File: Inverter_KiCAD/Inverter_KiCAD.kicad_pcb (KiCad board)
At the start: 2 copper layers, 184 x 186 mm, 172 parts, among them J101 Conn_02x19_Odd_Even, J102 Conn_01x03, J103 Conn_02x19_Odd_Even, J104 Conn_01x04, J1101 Conn_01x02, J1102 Conn_01x02, J501 PX0580-PC-12132, J801 USB_C_Receptacle_USB2.0, J802 Conn_01x05, J803 Conn_ST_STDC14, J804 Conn_01x04, J901 Conn_01x02, Q1101 SQ2310ES, Q201 HCPL-315J-500E, Q202 IRF540N, Q203 IRF540N, Q301 HCPL-315J-500E, Q302 IRF540N, Q303 IRF540N, Q401 HCPL-315J-500E, Q402 IRF540N, Q403 IRF540N, Q901 BUK9637-100E, SW801 SW_Push, SW802 SW_Push, SW803 SW_Push, SW804 SW_Push, SW805 SW_Push, U1201 TCN75A, U201 MPRB2415S-6W, U202 MPRB2415S-6W, U203 HCPL-7800-500E, U204 GO 10-SME/SP3, U301 MPRB2415S-6W, U302 MPRB2415S-6W, U303 HCPL-7800-500E, U304 GO 10-SME/SP3, U401 MPRB2415S-6W, U402 MPRB2415S-6W, U403 HCPL-7800-500E, U404 GO 10-SME/SP3, U501 MP-LD30-23B12R2, U502 173010542, U503 AZ1117-3.3, U601 GO 10-SME/SP3, U602 HCPL-7800-500E, U701 17791063215, U801 STM32G474RETx, U802 USBLC6-2SC6, U901 ACPL-077L, U902 TC1412, Y801 16M

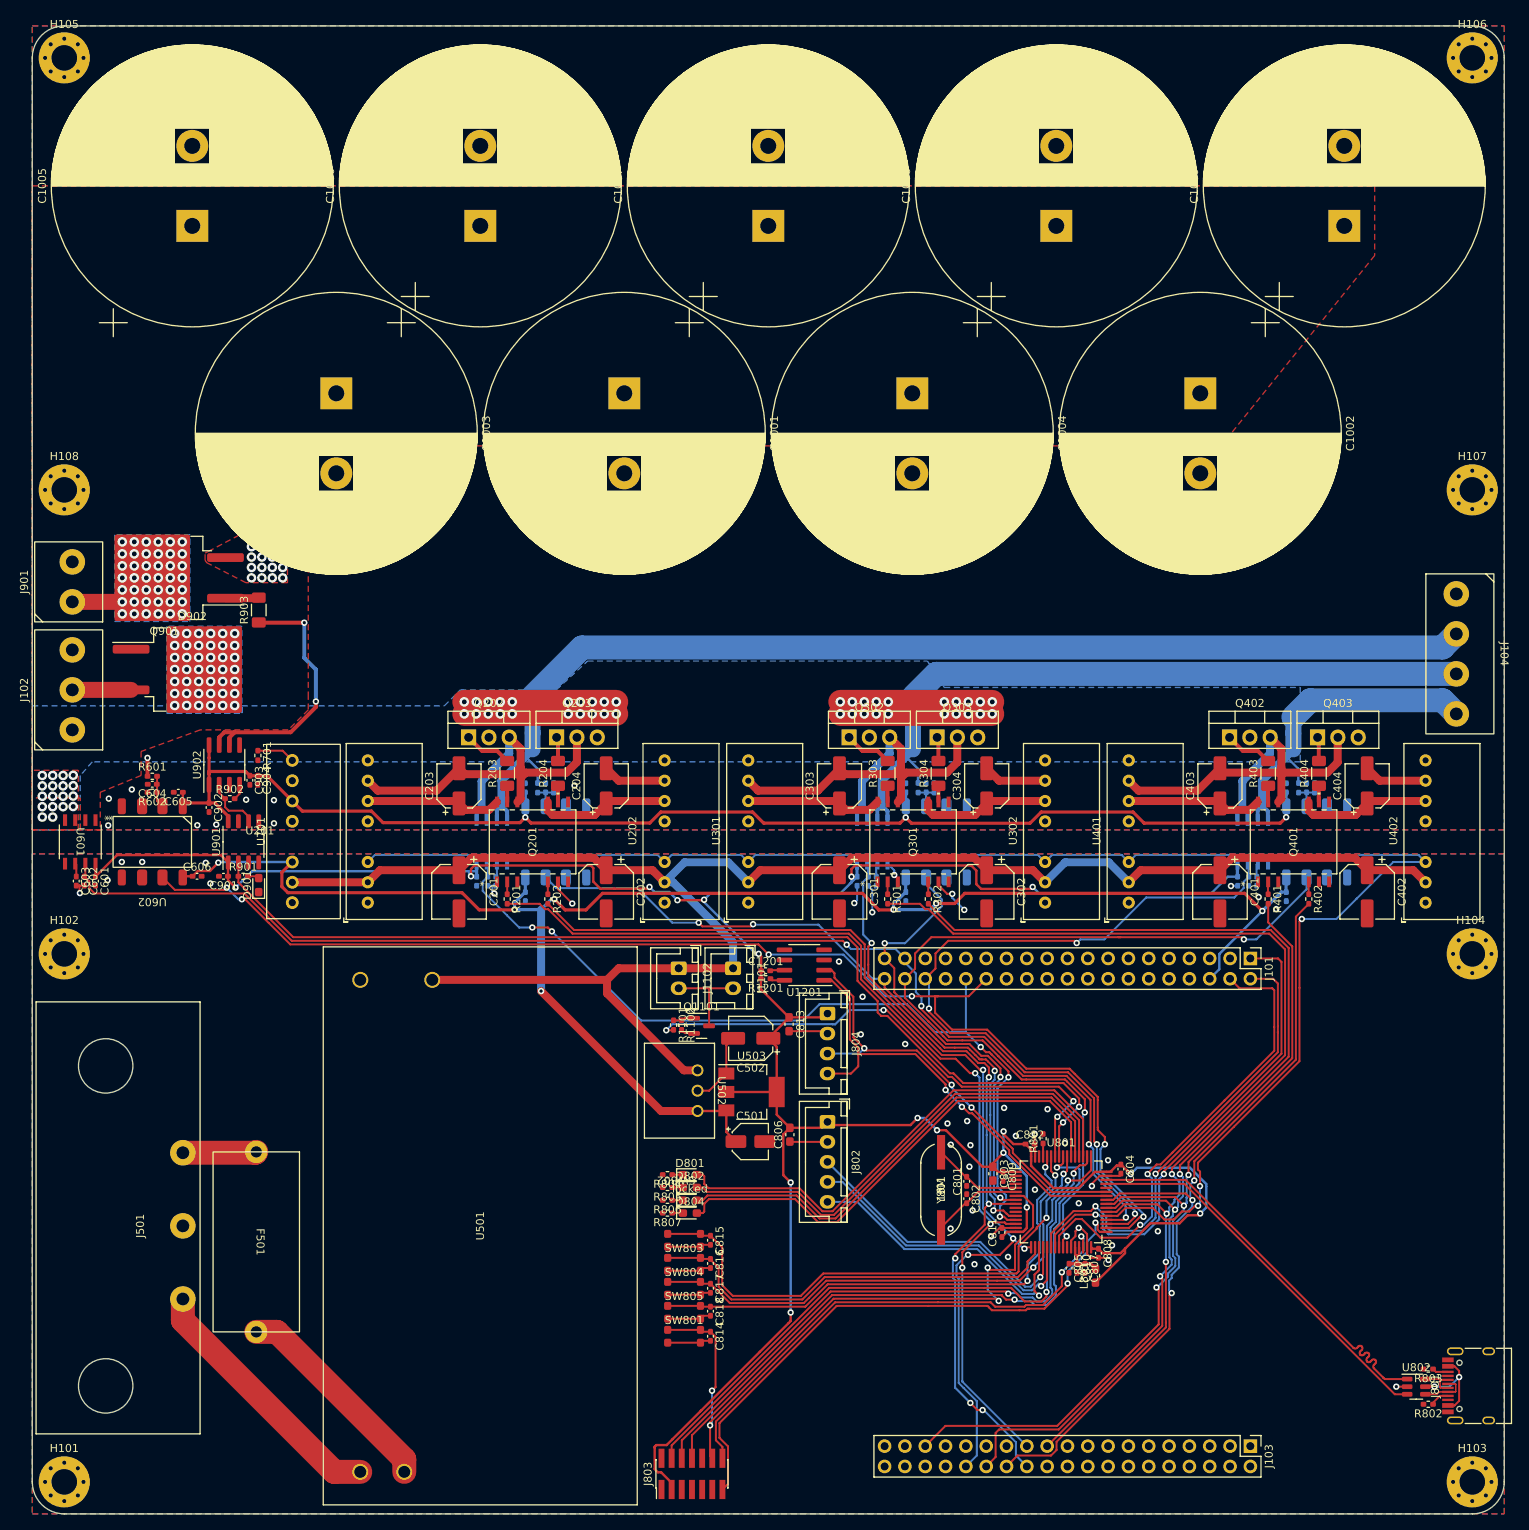
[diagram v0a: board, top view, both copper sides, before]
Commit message: change pcb
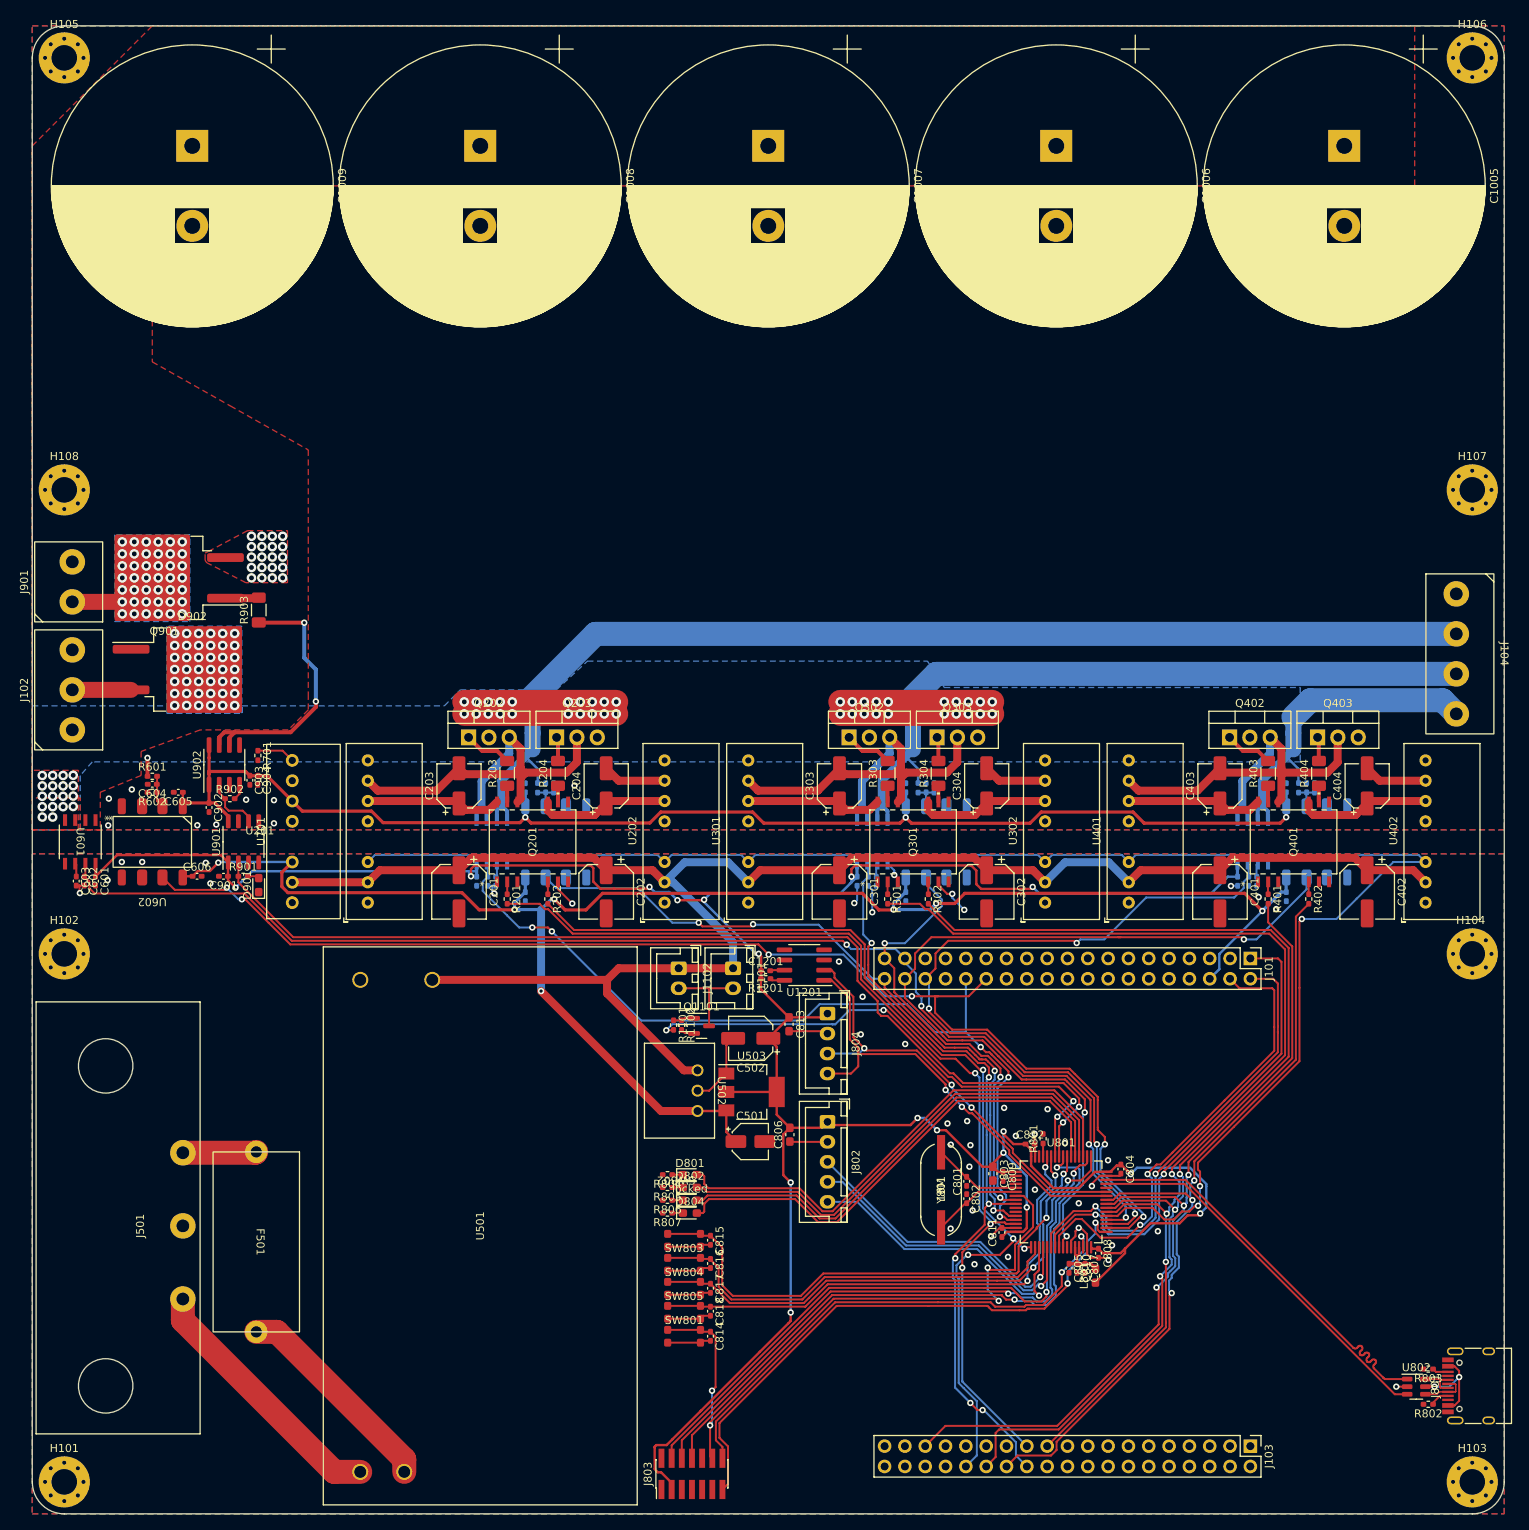
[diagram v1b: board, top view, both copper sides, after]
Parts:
- removed C1001, C1002, C1003, C1004: 1.5m, Capacitor_THT:CP_Radial_D35.0mm_P10.00mm_SnapIn
- moved C1005 144.3 mm to (197.0, 29.0), turned to -90 degrees
- moved C1009 144.3 mm to (53.0, 29.0), turned to -90 degrees
- moved C1006 72.7 mm to (161.0, 29.0), turned to -90 degrees
- moved C1008 72.7 mm to (89.0, 29.0), turned to -90 degrees
- moved C1007 10.0 mm to (125.0, 29.0), turned to -90 degrees
